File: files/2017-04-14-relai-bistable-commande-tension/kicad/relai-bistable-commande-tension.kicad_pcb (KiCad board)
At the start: 2 copper layers, 57.9 x 73.1 mm, 19 parts, among them T1 BC337, T2 BC337

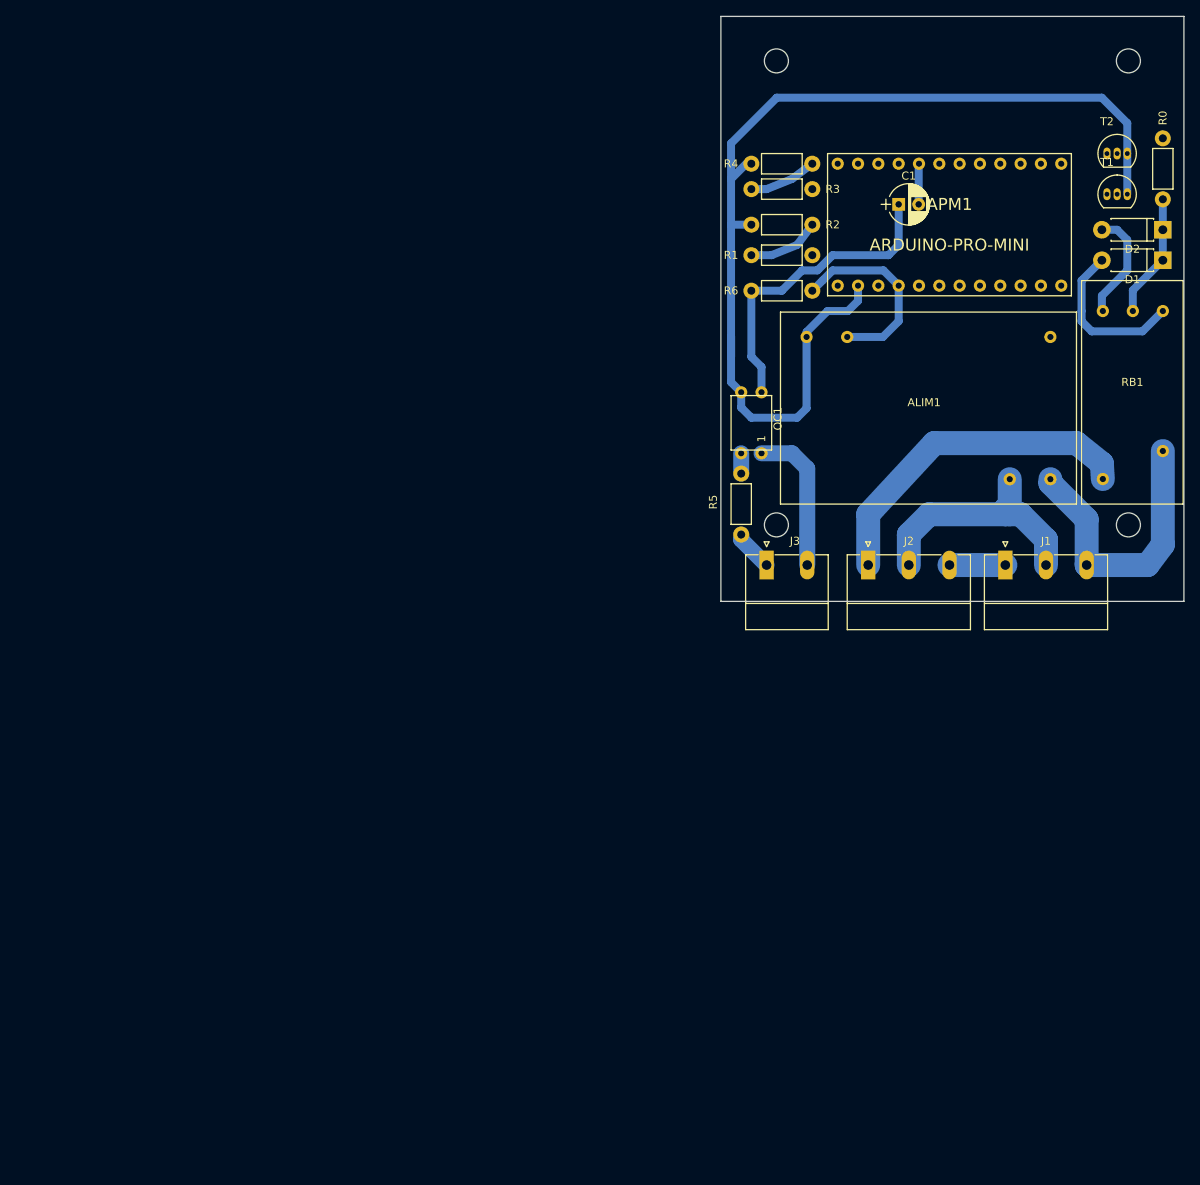
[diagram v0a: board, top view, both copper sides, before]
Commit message: premier jet du pcb
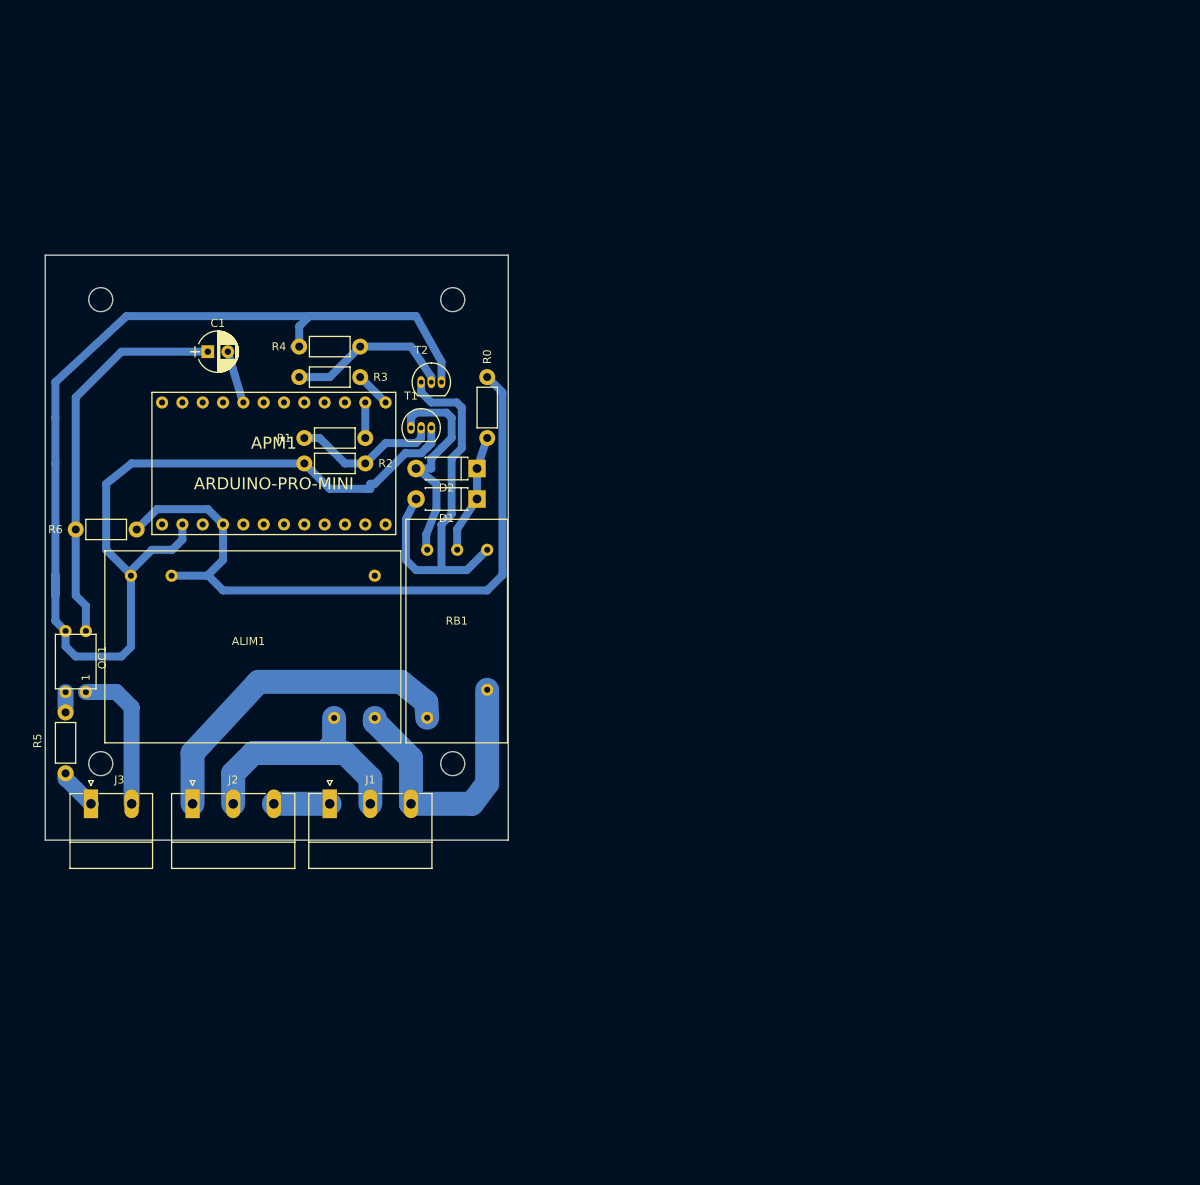
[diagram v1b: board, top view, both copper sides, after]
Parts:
- moved T1 91.8 mm to (123.8, 128.9)
- moved D1 90.8 mm to (132.1, 137.8)
- moved D2 90.8 mm to (132.1, 134.0)
- moved T2 90.4 mm to (125.1, 123.2)
- moved J3 89.6 mm to (83.8, 175.9)
- moved R0 89.6 mm to (133.3, 122.6)
- moved RB1 89.6 mm to (133.3, 144.1)
- moved J1 89.6 mm to (113.7, 175.9)
- moved J2 89.6 mm to (96.5, 175.9)
- moved R5 89.6 mm to (80.6, 172.1)
- moved R6 89.6 mm to (89.5, 141.6)
- moved ALIM1 89.6 mm to (122.6, 168.3)
- moved APM1 89.6 mm to (120.7, 133.3)
- moved OC1 89.6 mm to (83.2, 158.1)
- moved C1 88.3 mm to (98.4, 119.4)
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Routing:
- net GND: track 135.3 -> 204.3 mm
- net +3V3: track 24.6 -> 88.6 mm
- net Net-(D1-Pad2): track 20.4 -> 48.2 mm
- net Net-(D2-Pad2): track 14.0 -> 27.9 mm
- net Net-(R3-Pad2): track 8.50 -> 20.8 mm
- net Net-(C1-Pad1): track 39.1 -> 48.6 mm
- net Net-(R1-Pad1): track 9.13 -> 18.5 mm
- net Net-(APM1-Pad12): track 0.00 -> 4.49 mm
- net Net-(APM1-Pad11): track 0.00 -> 4.45 mm
- net Net-(APM1-Pad5): track 5.10 -> 6.72 mm
- net Net-(D1-Pad1): track 15.5 -> 14.9 mm

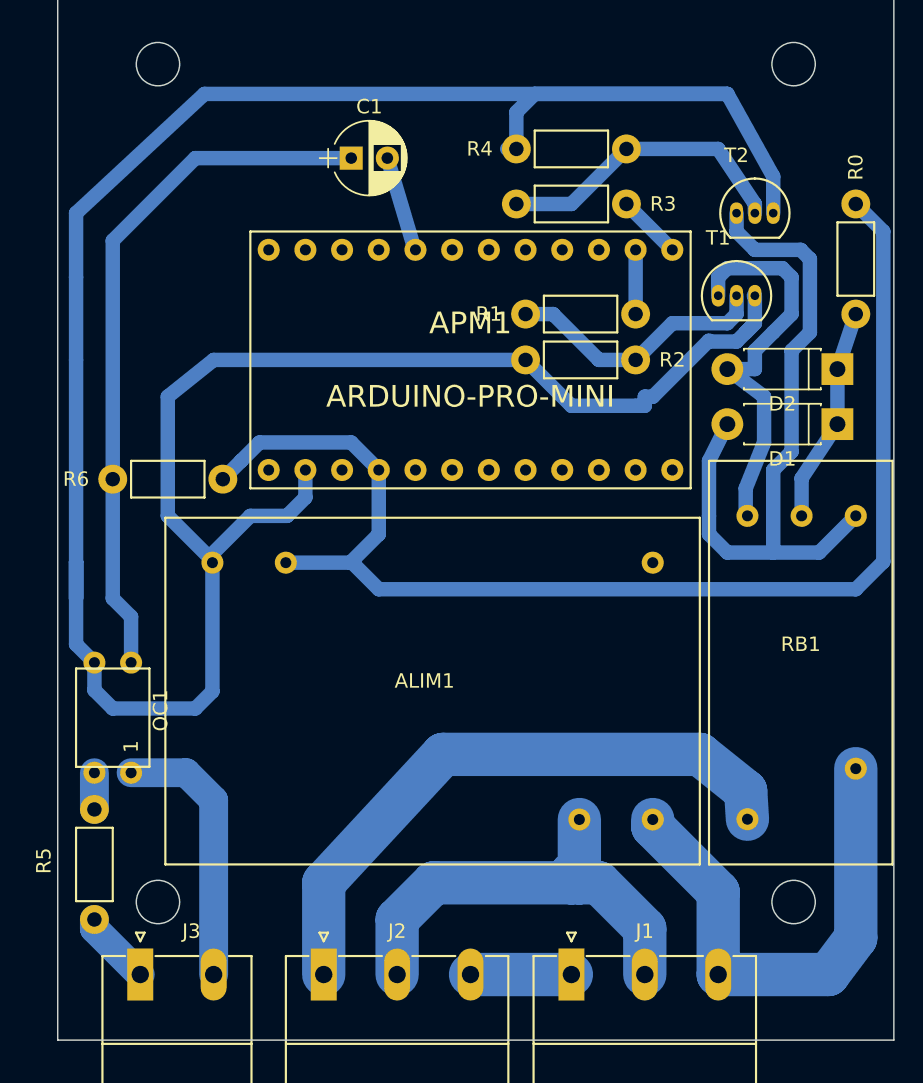
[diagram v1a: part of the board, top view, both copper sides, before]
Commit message: modif PCB Kicad
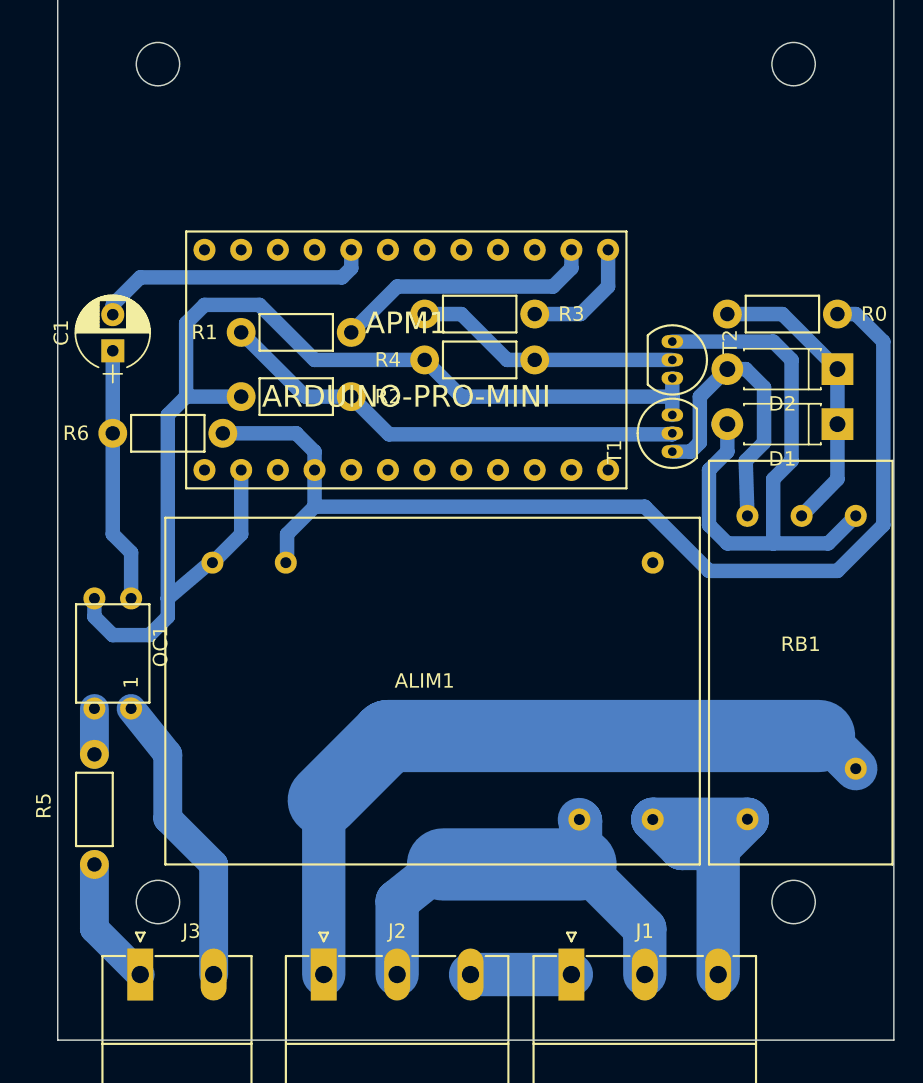
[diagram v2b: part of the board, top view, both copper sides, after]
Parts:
- moved C1 21.2 mm to (81.9, 132.7), turned to 90 degrees
- moved R2 19.8 mm to (98.4, 135.9)
- moved R1 19.7 mm to (90.8, 131.4)
- moved R4 15.9 mm to (103.5, 133.3)
- moved T1 11.3 mm to (120.7, 139.7), turned to 90 degrees
- moved T2 9.94 mm to (120.7, 132.1), turned to 270 degrees
- moved R3 9.92 mm to (111.1, 130.2)
- moved R0 7.73 mm to (132.1, 130.2), turned to 180 degrees
- moved OC1 4.45 mm to (83.2, 153.7)
- moved APM1 4.45 mm to (116.2, 133.3)
- moved R5 3.81 mm to (80.6, 168.3)
- moved R6 3.17 mm to (89.5, 138.4)
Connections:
- RB1 pad 3: Net-(J2-Pad1) -> AC
- RB1 pad 5: AC -> Net-(J2-Pad1)
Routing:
- net GND: track 204.3 -> 82.9 mm
- net Net-(C1-Pad1): track 48.6 -> 17.7 mm
- net Net-(R1-Pad1): track 18.5 -> 32.8 mm
- net Net-(APM1-Pad11): track 4.45 -> 18.4 mm
- net +3V3: track 88.6 -> 74.7 mm
- net Net-(APM1-Pad5): track 6.72 -> 19.6 mm
- net AC: track 35.1 -> 23.5 mm
- net Net-(J2-Pad1): track 42.3 -> 51.4 mm
- net Net-(D2-Pad2): track 27.9 -> 20.7 mm
- net Net-(D1-Pad2): track 48.2 -> 41.6 mm
- net Net-(D1-Pad1): track 14.9 -> 20.4 mm
- net Net-(APM1-Pad12): track 4.49 -> 8.41 mm
- net Net-(J3-Pad1): track 5.13 -> 8.94 mm
- net Net-(R3-Pad2): track 20.8 -> 18.5 mm
- net Net-(J3-Pad2): track 18.6 -> 20.6 mm
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
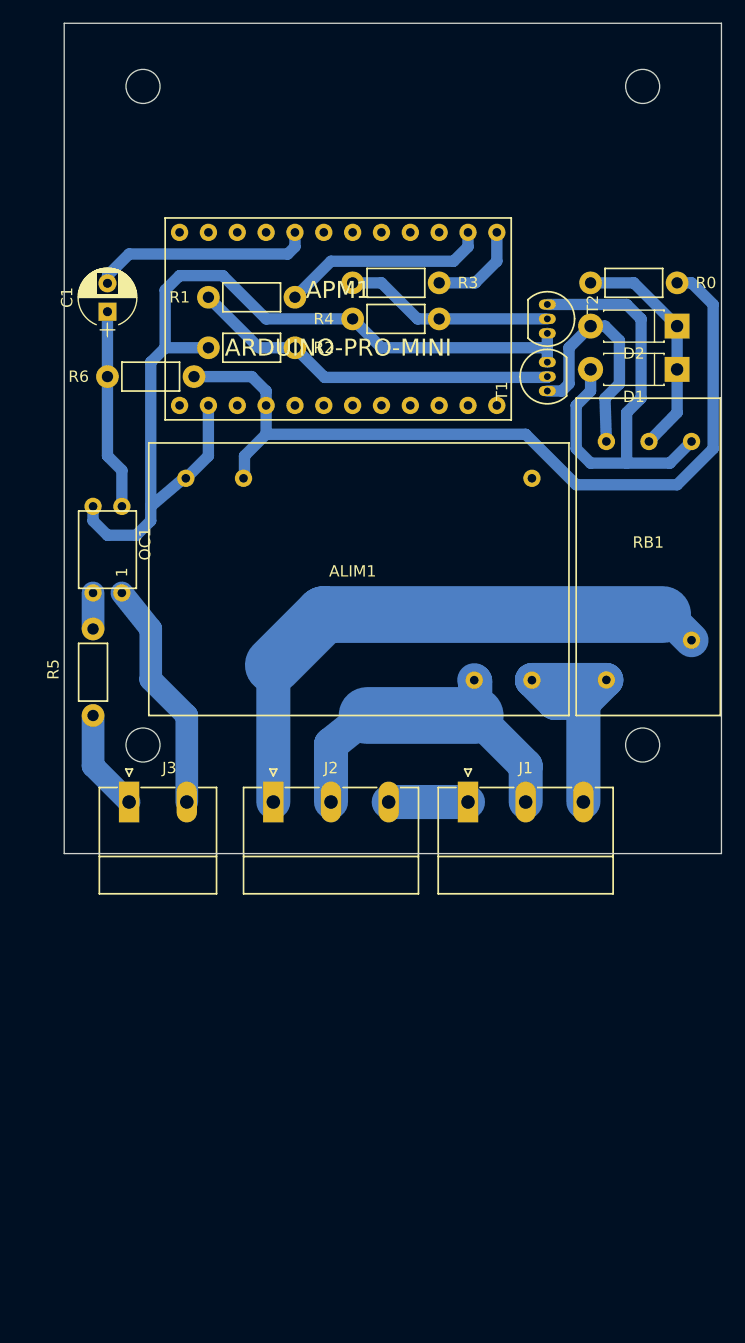
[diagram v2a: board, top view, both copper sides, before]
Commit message: pcb kicad
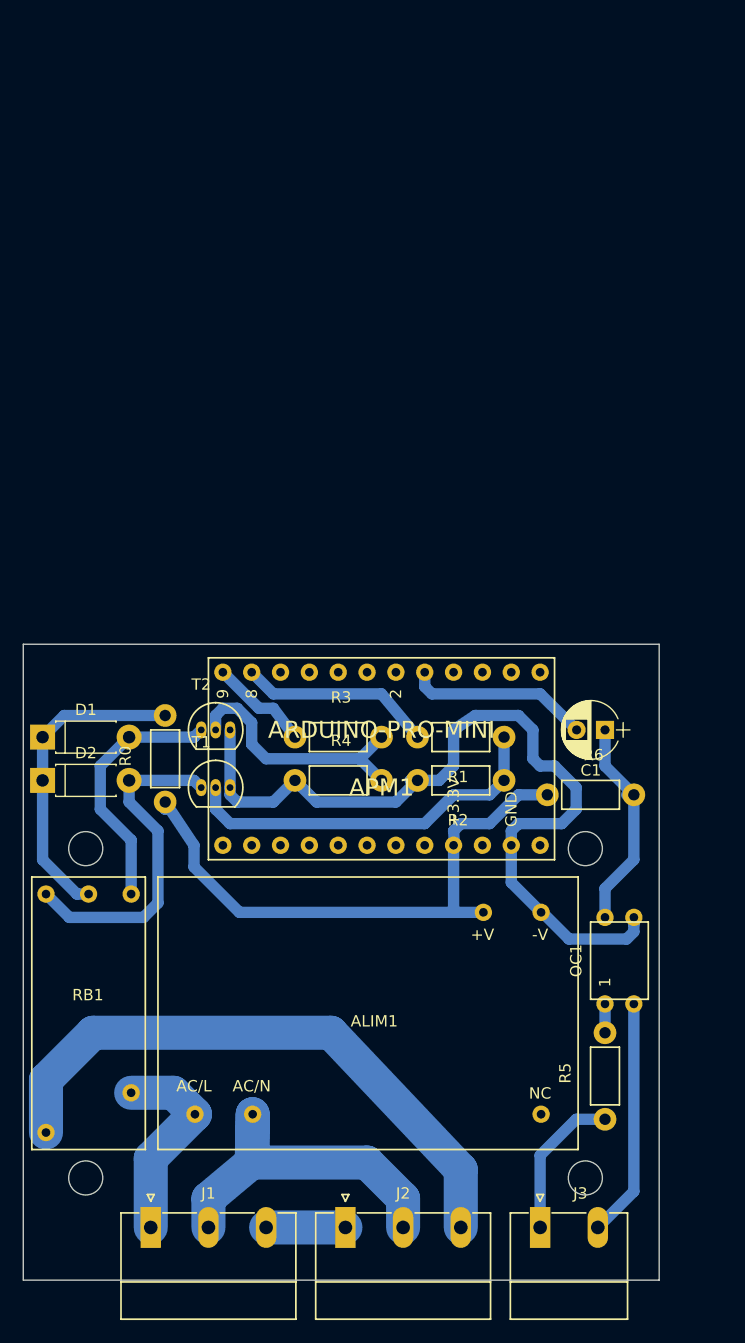
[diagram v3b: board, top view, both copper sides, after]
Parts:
- moved D2 68.7 mm to (76.2, 174.0), turned to 0 degrees
- moved D1 64.6 mm to (76.2, 170.2), turned to 0 degrees
- moved R0 64.2 mm to (87.0, 175.9), turned to 90 degrees
- moved RB1 63.4 mm to (84.0, 184.0)
- moved R5 57.4 mm to (125.7, 203.8)
- moved C1 57.2 mm to (125.7, 169.5), turned to 180 degrees
- moved OC1 55.9 mm to (125.7, 189.9), turned to 90 degrees
- moved J3 52.1 mm to (120.0, 213.4)
- moved T2 48.3 mm to (90.2, 169.5), turned to 0 degrees
- moved R6 48.2 mm to (120.7, 175.3), turned to 0 degrees
- moved J1 46.7 mm to (85.7, 213.4)
- moved R1 46.7 mm to (116.8, 170.2), turned to 180 degrees
- moved T1 46.4 mm to (90.2, 174.6), turned to 0 degrees
- moved APM1 45.6 mm to (92.1, 172.1), turned to 270 degrees
- moved R2 42.3 mm to (116.8, 174.0)
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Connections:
- J1 pad 1: Earth -> AC
- J1 pad 3: AC -> Earth
- J2 pad 1: Net-(J2-Pad1) -> Earth
- J2 pad 3: Earth -> Net-(J2-Pad3)
- OC1 pad 1: Net-(J3-Pad2) -> Net-(OC1-Pad1)
- OC1 pad 2: Net-(OC1-Pad2) -> Net-(J3-Pad2)
- R5 pad 2: Net-(OC1-Pad2) -> Net-(OC1-Pad1)
- RB1 pad 3: AC -> Net-(J2-Pad3)
- RB1 pad 5: Net-(J2-Pad1) -> AC
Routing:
- net Net-(J2-Pad3): track 0.00 -> 53.2 mm
- net Net-(J2-Pad1): track 51.4 -> 0.00 mm
- net +3V3: track 74.7 -> 51.7 mm
- net Net-(D1-Pad2): track 41.6 -> 22.6 mm
- net Net-(D2-Pad2): track 20.7 -> 29.7 mm
- net Net-(D1-Pad1): track 20.4 -> 27.7 mm
- net GND: track 82.9 -> 76.4 mm
- net AC: track 23.5 -> 18.0 mm
- net Net-(J3-Pad1): track 8.94 -> 13.4 mm
- net Net-(R3-Pad2): track 18.5 -> 22.6 mm
- net Net-(APM1-Pad5): track 19.6 -> 16.2 mm
- net Net-(OC1-Pad2): track 3.18 -> 0.00 mm
- net Net-(OC1-Pad1): track 0.00 -> 2.54 mm
- net Net-(ALIM1-Pad3): track 31.3 -> 33.2 mm
- net Net-(C1-Pad1): track 17.7 -> 19.2 mm
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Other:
- board size 57.9 x 73.1 mm -> 56 x 56 mm
- net class POWER removed
